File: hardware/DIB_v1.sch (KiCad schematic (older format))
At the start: 2 parts, among them J1 20-pin power socket, J3 28-pin module socket

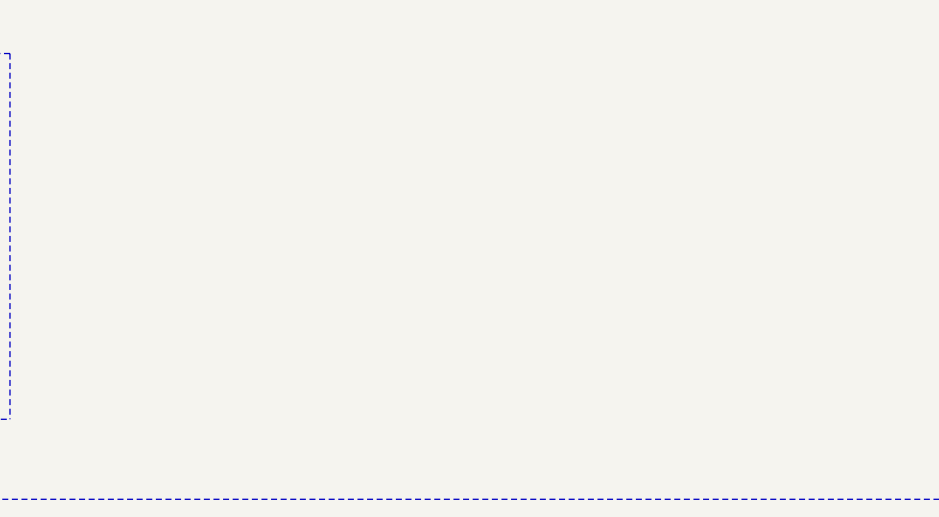
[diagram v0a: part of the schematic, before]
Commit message: Adding last known changes to shematics
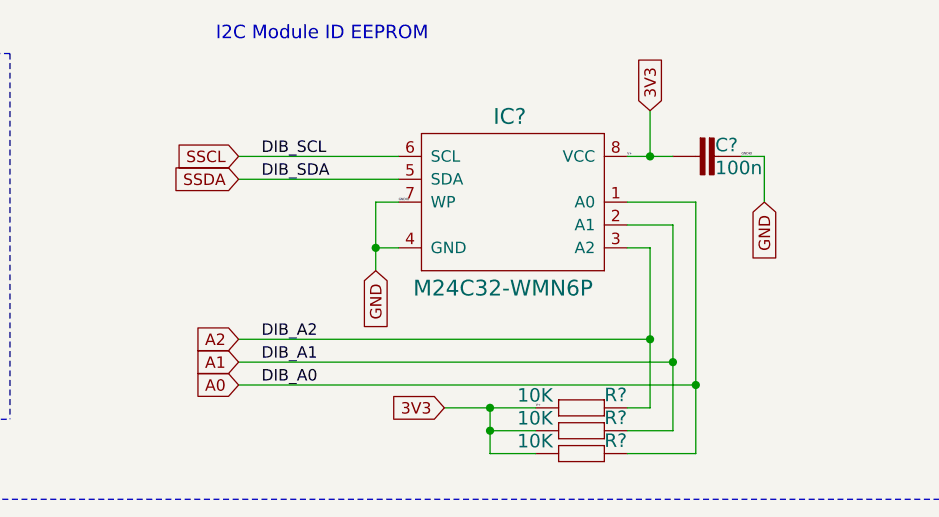
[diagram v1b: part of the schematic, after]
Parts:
- added C?: 100n, Capacitor_SMD:C_0603_1608Metric, symbol LCD_PMOD-rescue:C-EUC0603-EEZ_DIB_DCM220_r2B7-eagle-import
- added IC?: M24C32-WMN6P, OPA2211:SOIC127P600X170-9N, symbol LCD_PMOD-rescue:AT24CXXSOIC8-EEZ_DIB_DCM220_r2B7-eagle-import
- added R? (x3): 10K, Capacitor_SMD:C_0805_2012Metric, symbol LCD_PMOD-rescue:R-EU_R0805-EEZ_DIB_DCM220_r2B7-eagle-import
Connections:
- net A0: now also IC?.1 (A0), R?.2
- net A1: now also IC?.2 (A1), R?.2
- net A2: now also IC?.3 (A2), R?.2
- net GND: now also C?.1, IC?.4 (GND), IC?.7 (WP)
- net SSCL: now also IC?.6 (SCL)
- net SSDA: now also IC?.5 (SDA)
- new net 3V3: C?.2, IC?.8 (VCC), R?.1, R?.1, R?.1
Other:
- note added: "I2C Module ID EEPROM"
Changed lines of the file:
@@
 $Descr A4 11693 8268
 encoding utf-8
-Sheet 4 11
+Sheet 4 10
 Title ""
-Date ""
-Rev ""
-Comp ""
+Date "2020-01-29"
+Rev "0.1"
+Comp "Envox d.o.o."
 Comment1 ""
 Comment2 ""
@@
 Wire Notes Line
 	6700 900  6700 2500
+Wire Wire Line
+	9400 1550 9700 1550
+Wire Wire Line
+	9700 1550 9700 2350
+Wire Wire Line
+	9700 2350 9700 2650
+Wire Wire Line
+	9700 2650 9400 2650
+Text Label 7800 2350 0    50   ~ 0
+DIB_A0
+Connection ~ 9700 2350
+Wire Wire Line
+	9400 1650 9600 1650
+Wire Wire Line
+	9600 1650 9600 2250
+Wire Wire Line
+	9600 2250 9600 2550
+Wire Wire Line
+	9600 2550 9400 2550
+Text Label 7800 2250 0    50   ~ 0
+DIB_A1
+Connection ~ 9600 2250
+Wire Wire Line
+	9400 1750 9500 1750
+Wire Wire Line
+	9500 1750 9500 2150
+Wire Wire Line
+	9500 2150 9500 2450
+Wire Wire Line
+	9500 2450 9400 2450
+Text Label 7800 2150 0    50   ~ 0
+DIB_A2
+Connection ~ 9500 2150
+Text Label 7800 1350 0    50   ~ 0
+DIB_SCL
+Text Label 7800 1450 0    50   ~ 0
+DIB_SDA
+Wire Wire Line
+	8400 1550 8300 1550
+Wire Wire Line
+	8300 1550 8300 1750
+Wire Wire Line
+	8300 1750 8400 1750
+Wire Wire Line
+	8300 1850 8300 1750
+Connection ~ 8300 1750
+Text Label 8400 1550 0    10   ~ 0
+GNDIO
+Wire Wire Line
+	9900 1350 10000 1350
+Text Label 9900 1350 0    10   ~ 0
+GNDIO
+Wire Wire Line
+	9400 1350 9500 1350
+Wire Wire Line
+	9600 1350 9500 1350
+Connection ~ 9500 1350
+Text Label 9400 1350 0    10   ~ 0
+V+
+Wire Wire Line
+	9000 2450 8800 2450
+Wire Wire Line
+	8800 2450 8800 2550
+Wire Wire Line
+	8800 2550 8800 2650
+Wire Wire Line
+	8800 2650 9000 2650
+Wire Wire Line
+	9000 2550 8800 2550
+Connection ~ 8800 2550
+Connection ~ 8800 2450
+Text Label 9000 2450 0    10   ~ 0
+V+
+$Comp
+L LCD_PMOD-rescue:C-EUC0603-EEZ_DIB_DCM220_r2B7-eagle-import C?
+U 1 0 5E650AE0
+P 9800 1350
+AR Path="/5E650AE0" Ref="C?"  Part="1"
+AR Path="/5E155363/5E650AE0" Ref="C?"  Part="1"
+AR Path="/5E500AA4/5E650AE0" Ref="C?"  Part="1"
+AR Path="/5E22C9F9/5E650AE0" Ref="C?"  Part="1"
+F 0 "C?" V 9785 1335 59  0000 L BNN
+F 1 "100n" V 9885 1335 59  0000 L BNN
+F 2 "Capacitor_SMD:C_0603_1608Metric" H 9800 1350 50  0001 C CNN
+F 3 "" H 9800 1350 50  0001 C CNN
+	1    9800 1350
+	0    1    1    0
+$EndComp
+$Comp
+L LCD_PMOD-rescue:R-EU_R0805-EEZ_DIB_DCM220_r2B7-eagle-import R?
+U 1 0 5E650AE7
+P 9200 2450
+AR Path="/5E650AE7" Ref="R?"  Part="1"
+AR Path="/5E155363/5E650AE7" Ref="R?"  Part="1"
+AR Path="/5E500AA4/5E650AE7" Ref="R?"  Part="1"
+AR Path="/5E22C9F9/5E650AE7" Ref="R?"  Part="1"
+F 0 "R?" H 9300 2359 59  0000 L BNN
+F 1 "10K" H 9075 2430 59  0000 R TNN
+F 2 "Capacitor_SMD:C_0805_2012Metric" H 9200 2450 50  0001 C CNN
+F 3 "" H 9200 2450 50  0001 C CNN
+	1    9200 2450
+	1    0    0    1
+$EndComp
+$Comp
+L LCD_PMOD-rescue:R-EU_R0805-EEZ_DIB_DCM220_r2B7-eagle-import R?
+U 1 0 5E650AEE
+P 9200 2550
+AR Path="/5E650AEE" Ref="R?"  Part="1"
+AR Path="/5E155363/5E650AEE" Ref="R?"  Part="1"
+AR Path="/5E500AA4/5E650AEE" Ref="R?"  Part="1"
+AR Path="/5E22C9F9/5E650AEE" Ref="R?"  Part="1"
+F 0 "R?" H 9300 2459 59  0000 L BNN
+F 1 "10K" H 9075 2530 59  0000 R TNN
+F 2 "Capacitor_SMD:C_0805_2012Metric" H 9200 2550 50  0001 C CNN
+F 3 "" H 9200 2550 50  0001 C CNN
+	1    9200 2550
+	1    0    0    1
+$EndComp
+$Comp
+L LCD_PMOD-rescue:R-EU_R0805-EEZ_DIB_DCM220_r2B7-eagle-import R?
+U 1 0 5E650AF5
+P 9200 2650
+AR Path="/5E650AF5" Ref="R?"  Part="1"
+AR Path="/5E155363/5E650AF5" Ref="R?"  Part="1"
+AR Path="/5E500AA4/5E650AF5" Ref="R?"  Part="1"
+AR Path="/5E22C9F9/5E650AF5" Ref="R?"  Part="1"
+F 0 "R?" H 9300 2559 59  0000 L BNN
+F 1 "10K" H 9075 2630 59  0000 R TNN
+F 2 "Capacitor_SMD:C_0805_2012Metric" H 9200 2650 50  0001 C CNN
+F 3 "" H 9200 2650 50  0001 C CNN
+	1    9200 2650
+	1    0    0    1
+$EndComp
+$Comp
+L LCD_PMOD-rescue:AT24CXXSOIC8-EEZ_DIB_DCM220_r2B7-eagle-import IC?
+U 1 0 5E650AFC
+P 8900 1550
+AR Path="/5E650AFC" Ref="IC?"  Part="1"
+AR Path="/5E155363/5E650AFC" Ref="IC?"  Part="1"
+AR Path="/5E500AA4/5E650AFC" Ref="IC?"  Part="1"
+AR Path="/5E22C9F9/5E650AFC" Ref="IC?"  Part="1"
+F 0 "IC?" H 8814 1884 69  0000 L BNN
+F 1 "M24C32-WMN6P" H 8464 1133 69  0000 L BNN
+F 2 "OPA2211:SOIC127P600X170-9N" H 8900 1550 50  0001 C CNN
+F 3 "" H 8900 1550 50  0001 C CNN
+	1    8900 1550
+	1    0    0    -1
+$EndComp
+Text Notes 7600 850  0    59   ~ 0
+I2C Module ID EEPROM
+Text GLabel 7700 1450 0    50   Input ~ 0
+SSDA
+Wire Wire Line
+	7700 1450 8400 1450
+Text GLabel 7700 1350 0    50   Input ~ 0
+SSCL
+Wire Wire Line
+	7700 1350 8400 1350
+Text GLabel 7700 2350 0    50   Input ~ 0
+A0
+Text GLabel 7700 2250 0    50   Input ~ 0
+A1
+Text GLabel 7700 2150 0    50   Input ~ 0
+A2
+Wire Wire Line
+	7700 2150 9500 2150
+Wire Wire Line
+	7700 2250 9600 2250
+Wire Wire Line
+	7700 2350 9700 2350
+Text GLabel 10000 1550 3    50   Input ~ 0
+GND
+Wire Wire Line
+	10000 1350 10000 1550
+Text GLabel 8300 1850 3    50   Input ~ 0
+GND
+Text GLabel 9500 1150 1    50   Input ~ 0
+3V3
+Text GLabel 8600 2450 0    50   Input ~ 0
+3V3
+Wire Wire Line
+	9500 1150 9500 1350
+Wire Wire Line
+	8600 2450 8800 2450
 $EndSCHEMATC
